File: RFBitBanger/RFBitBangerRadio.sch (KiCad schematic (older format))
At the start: 144 parts, among them J12 Conn_Coaxial, Q1 2N3904, Q10 2N3904, Q11 2N3904, Q12 2N3904, Q13 2N2907, Q2 2N3904, Q3 2N2222, Q5 2N2222, Q6 2N2222, Q7 2N2222, Q8 2N2907, Q9 2N3904, T1 Trifilar, T2 Trifilar, T3 Current, U4 LM358, U6 SI5351A, Y2 7.023 MHz, Y3 27 MHz, Y4 7.023 MHz

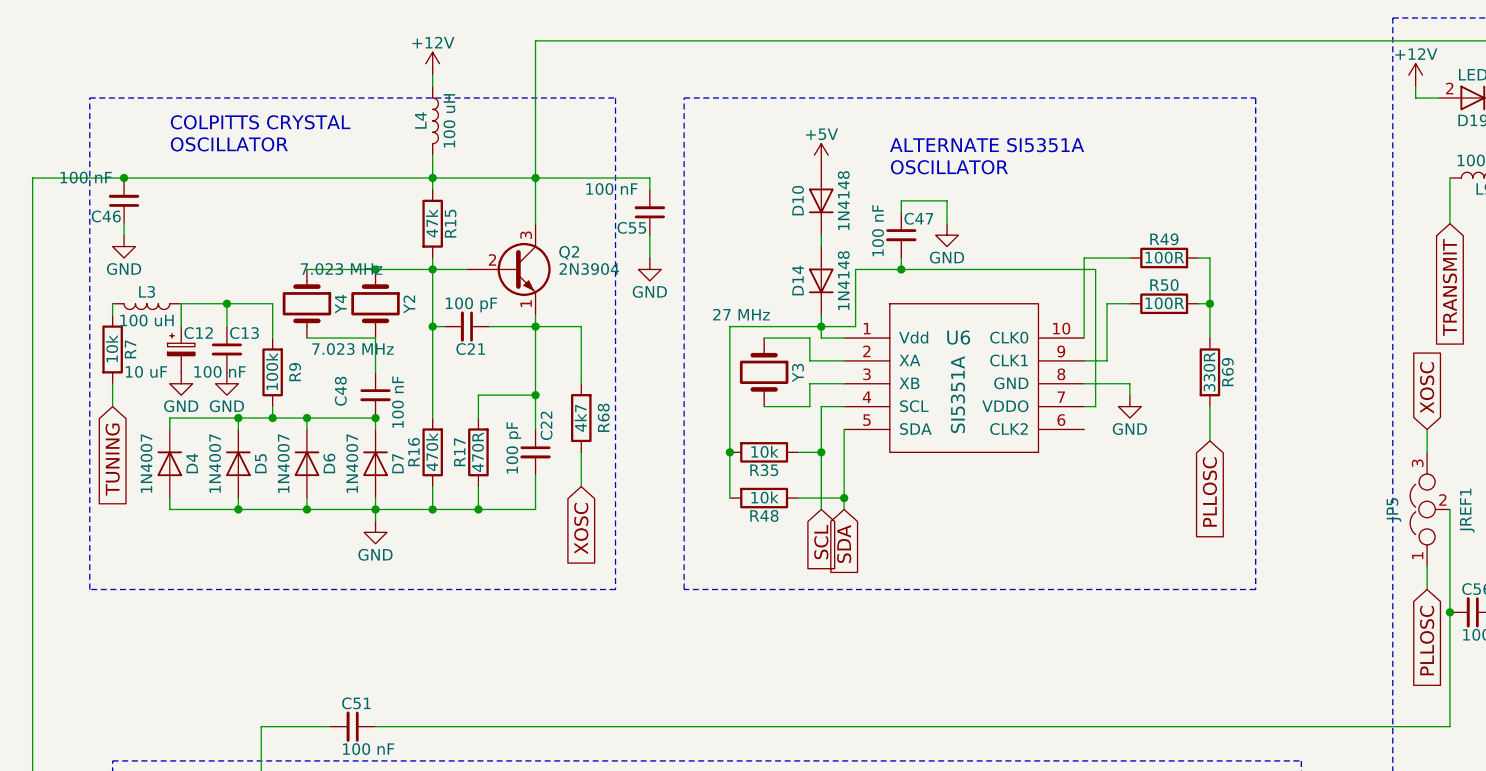
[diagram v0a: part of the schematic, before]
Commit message: Made 3 crystals instead of 2
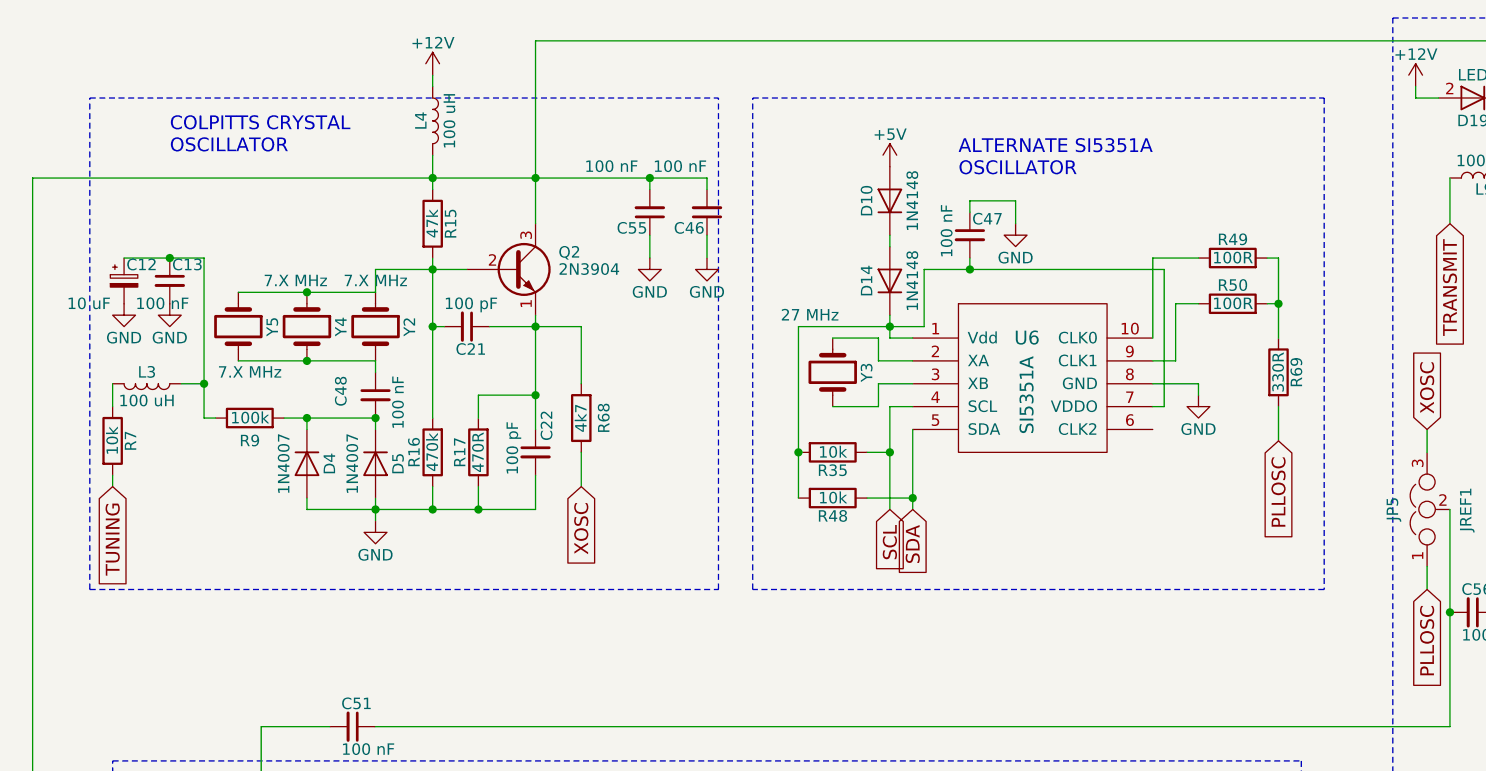
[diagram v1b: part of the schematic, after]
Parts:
- removed D4, D5: 1N4007, Diodes_THT:D_DO-41_SOD81_P7.62mm_Horizontal, symbol D
- added Y5: 7.X MHz, Crystals:Crystal_HC49-U_Vertical, symbol Crystal
- C27: footprint Capacitors_THT:C_Disc_D5.0mm_W2.5mm_P2.50mm -> Capacitors_THT:C_Disc_D5.0mm_W2.5mm_P5.00mm
- Y2, Y4: value 7.023 MHz -> 7.X MHz
- renumbered D6 to D4, D7 to D5
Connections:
- net at C12.1, C13.1, L3.1: now also R9.1; no longer R9.2
- net at C21.2, Q2.2 (B), R15.2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: now also Y5.1
- net at C48.2, D4.1 (K), D5.1 (K): now also R9.2; no longer R9.1
- net at C48.1, Y2.2, Y4.2: now also Y5.2
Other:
- moved on the sheet: C12, C13, C46, C47, D10, D14, L3, R35, R48, R49, R50, R69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
